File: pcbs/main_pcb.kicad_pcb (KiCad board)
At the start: 2 copper layers, 139.3 x 147.8 mm, 60 parts

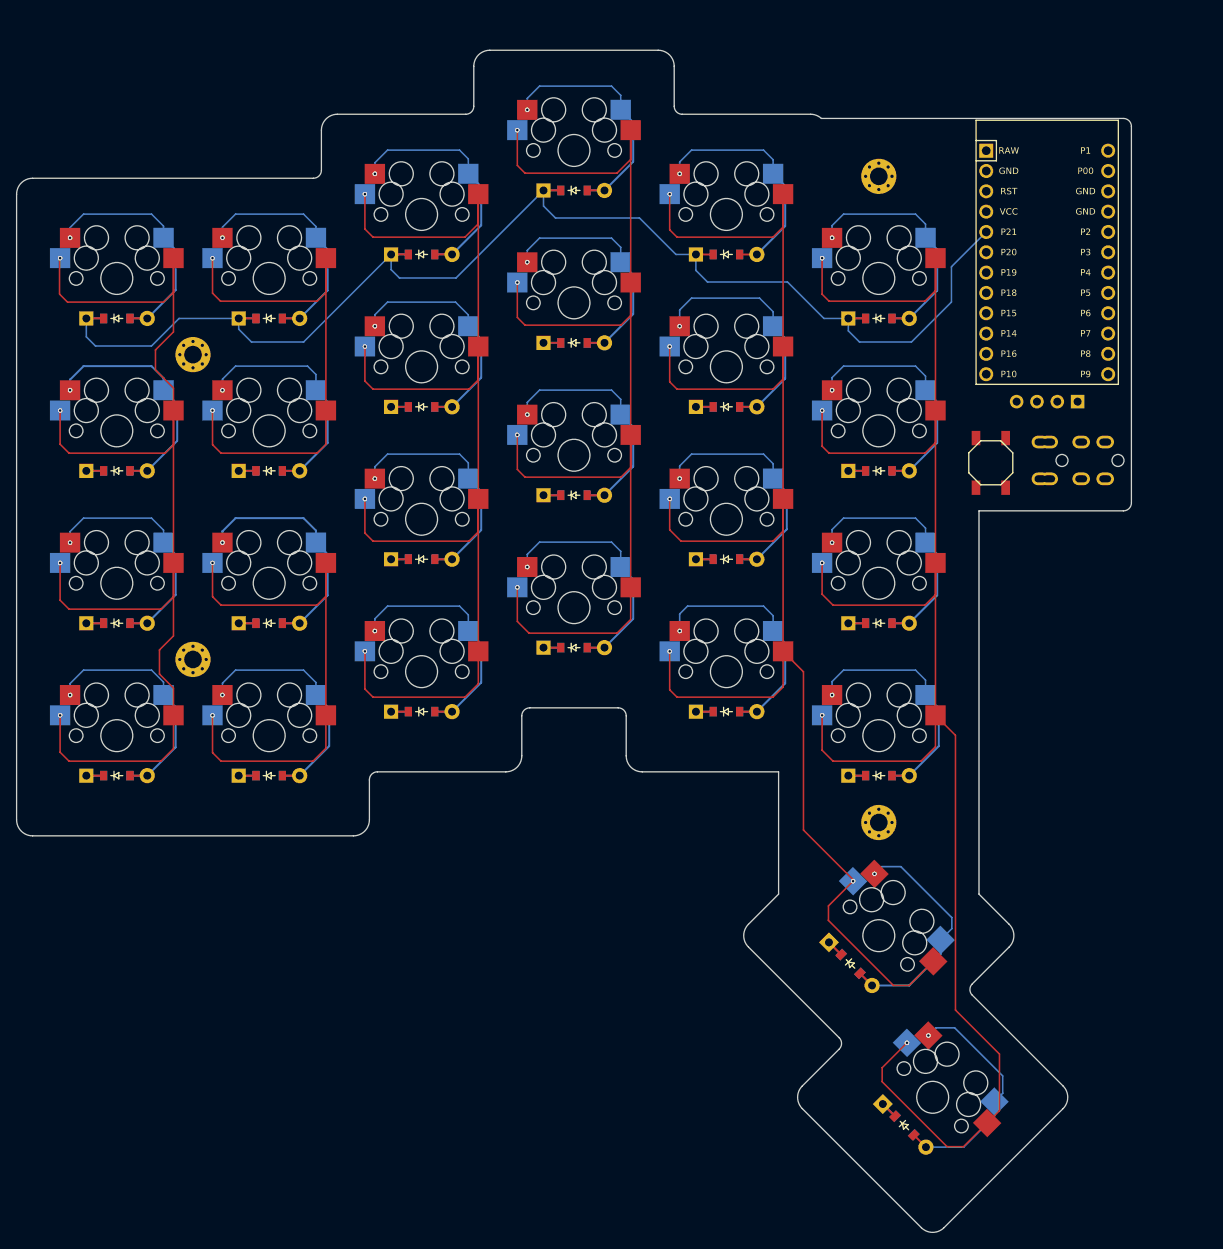
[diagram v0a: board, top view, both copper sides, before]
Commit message: att
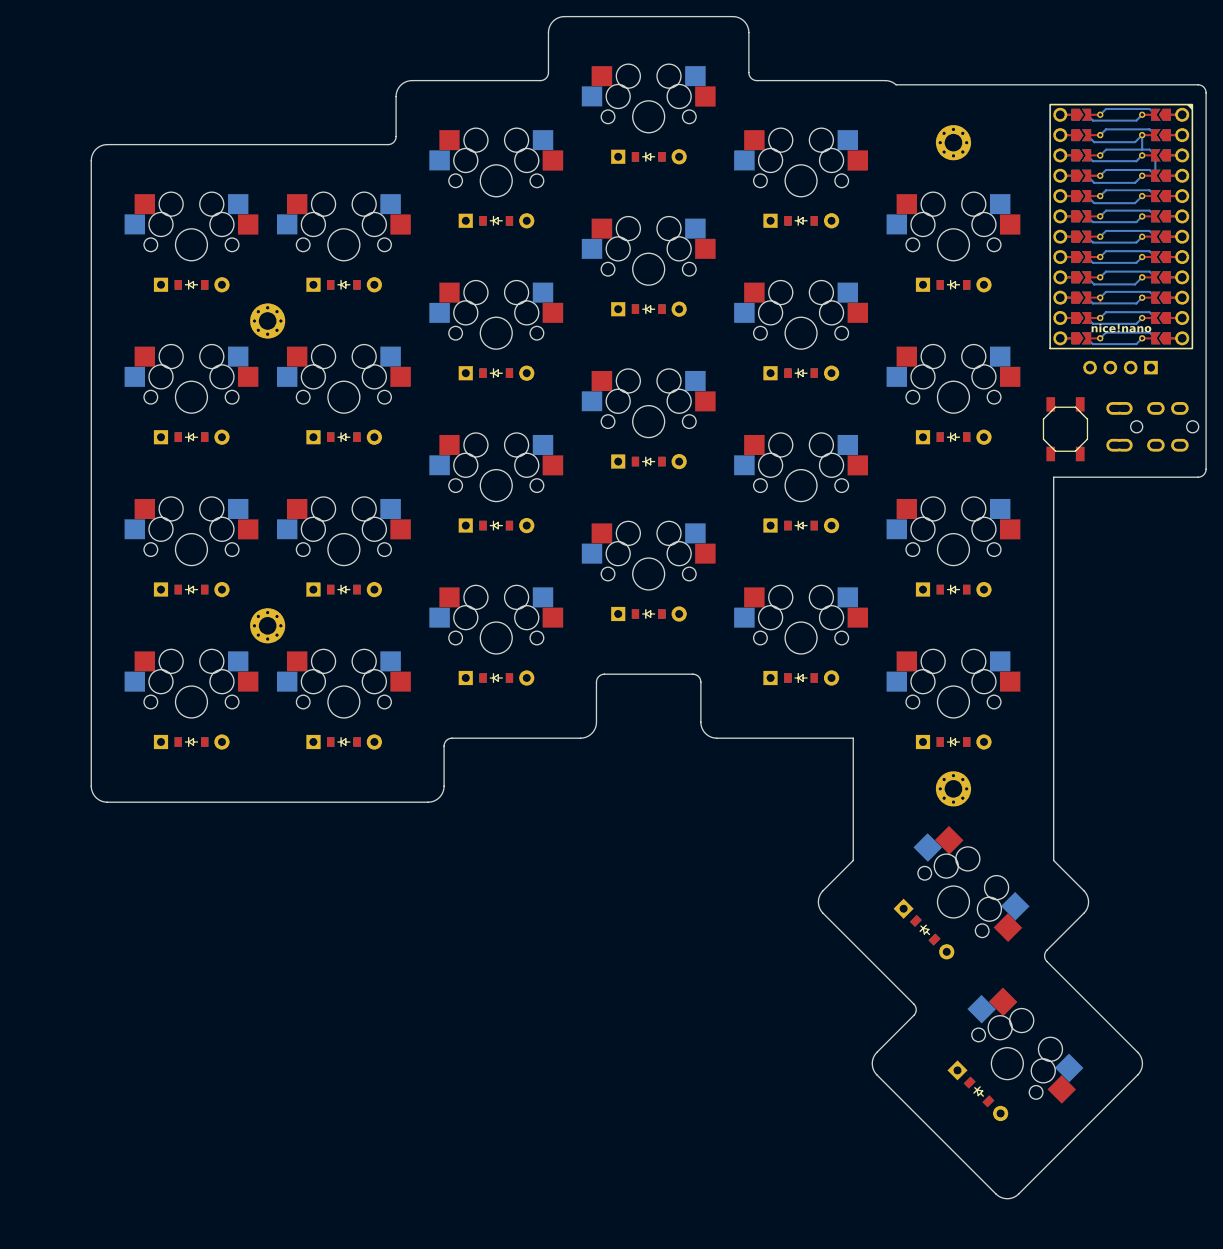
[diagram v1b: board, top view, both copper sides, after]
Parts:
- MCU1: value (none) -> nice!nano_v2; footprint ProMicro -> nice!nano_v2
- moved MCU1 10.3 mm to (266.2, 90.6), turned to 0 degrees
- moved TRRS1 10.2 mm to (276.8, 117.9)
- moved S2 10.2 mm to (150.0, 130.9)
- moved D7 10.2 mm to (169.1, 116.9)
- moved S13 10.2 mm to (207.2, 134.0)
- moved _2 10.2 mm to (159.5, 140.5)
- moved D20 10.2 mm to (226.2, 89.8)
- moved S15 10.2 mm to (207.2, 95.9)
- moved D11 10.2 mm to (188.1, 108.9)
- moved D23 10.2 mm to (245.2, 116.9)
- moved S21 10.2 mm to (245.2, 150.0)
- moved D1 10.2 mm to (150.0, 155.0)
- moved B1 10.2 mm to (259.2, 115.9)
- moved D15 10.2 mm to (207.2, 100.9)
- moved D9 10.2 mm to (188.1, 147.0)
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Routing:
- net P9: track 230.1 -> 9.13 mm, vias 5 -> 0
- net P8: track 208.2 -> 9.13 mm, vias 5 -> 0
- net P21: track 173.9 -> 9.26 mm
- net P14: track 156.3 -> 9.20 mm, vias 4 -> 0
- net P10: track 151.6 -> 9.13 mm, vias 4 -> 0
- net P7: track 151.7 -> 9.74 mm, vias 4 -> 0
- net P16: track 132.9 -> 9.20 mm, vias 4 -> 0
- net inner_num: track 33.3 -> 0.00 mm, vias 1 -> 0
- net inner_bottom: track 33.1 -> 0.00 mm, vias 1 -> 0
- net aditional_bottom: track 32.9 -> 0.00 mm, vias 1 -> 0
- net middle_bottom: track 32.9 -> 0.00 mm, vias 1 -> 0
- net inner_home: track 32.9 -> 0.00 mm, vias 1 -> 0
- net pinky_top: track 32.9 -> 0.00 mm, vias 1 -> 0
- net index_bottom: track 32.9 -> 0.00 mm, vias 1 -> 0
- net middle_home: track 32.8 -> 0.00 mm, vias 1 -> 0
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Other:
- outline, holes or cut-outs redrawn
